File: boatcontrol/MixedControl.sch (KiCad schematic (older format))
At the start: 12 parts, among them J2401 Conn_01x01_Male, J2402 Conn_01x01_Male, J2403 Conn_02x20_Odd_Even Socket, U2401 MCP23017-E/SP

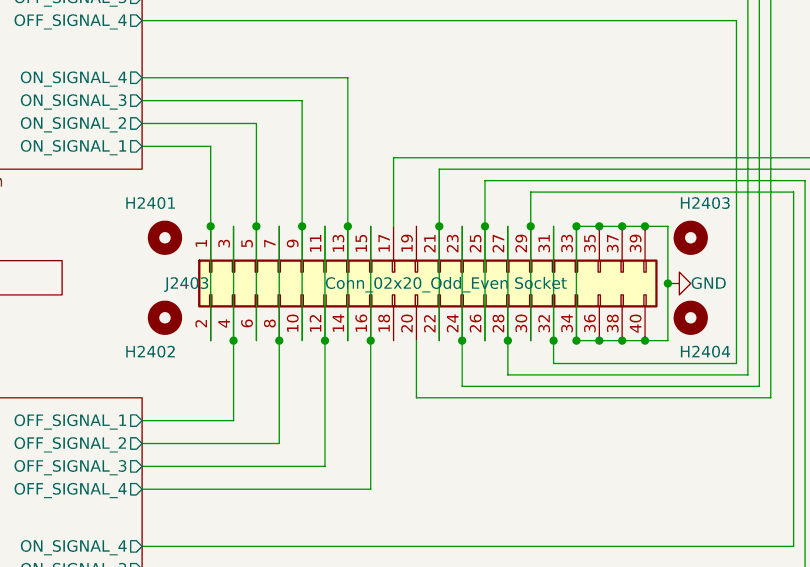
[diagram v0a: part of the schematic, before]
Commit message: interrim
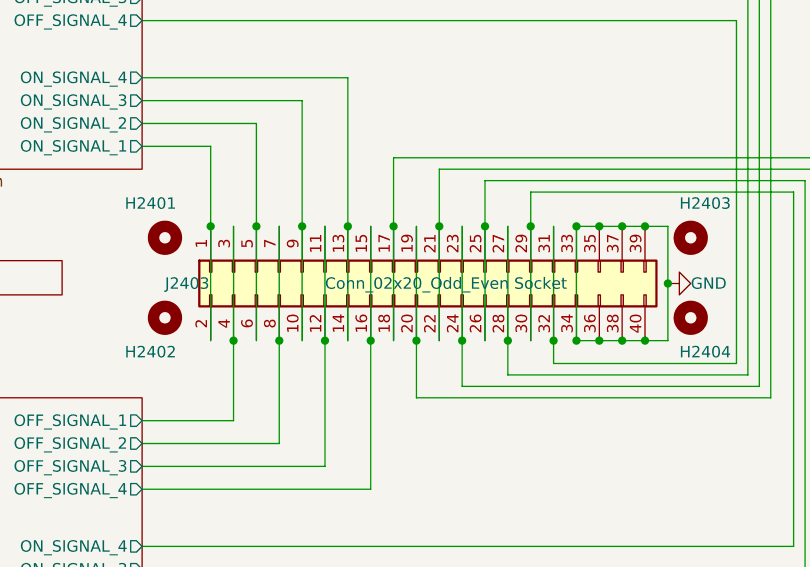
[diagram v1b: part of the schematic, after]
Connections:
- net MixedBlock1/OFF_SIGNAL_1: now also J2403.19 (Pin_19)
- net MixedBlock2/ON_SIGNAL_1: now also J2403.18 (Pin_18)
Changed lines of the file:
@@
 	7650 3600 7650 4100
 Connection ~ 7650 3600
+Wire Wire Line
+	8450 4100 8450 3600
+Connection ~ 8450 3600
+Wire Wire Line
+	8550 3600 8550 4100
+Connection ~ 8550 4100
 $EndSCHEMATC
